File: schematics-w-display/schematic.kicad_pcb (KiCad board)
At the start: 2 copper layers, 59.8 x 61.5 mm, 8 parts, among them J1 Conn_01x21_Female, J2 Conn_01x06_Female, J3 Conn_01x21_Female, J4 Conn_01x08_Female

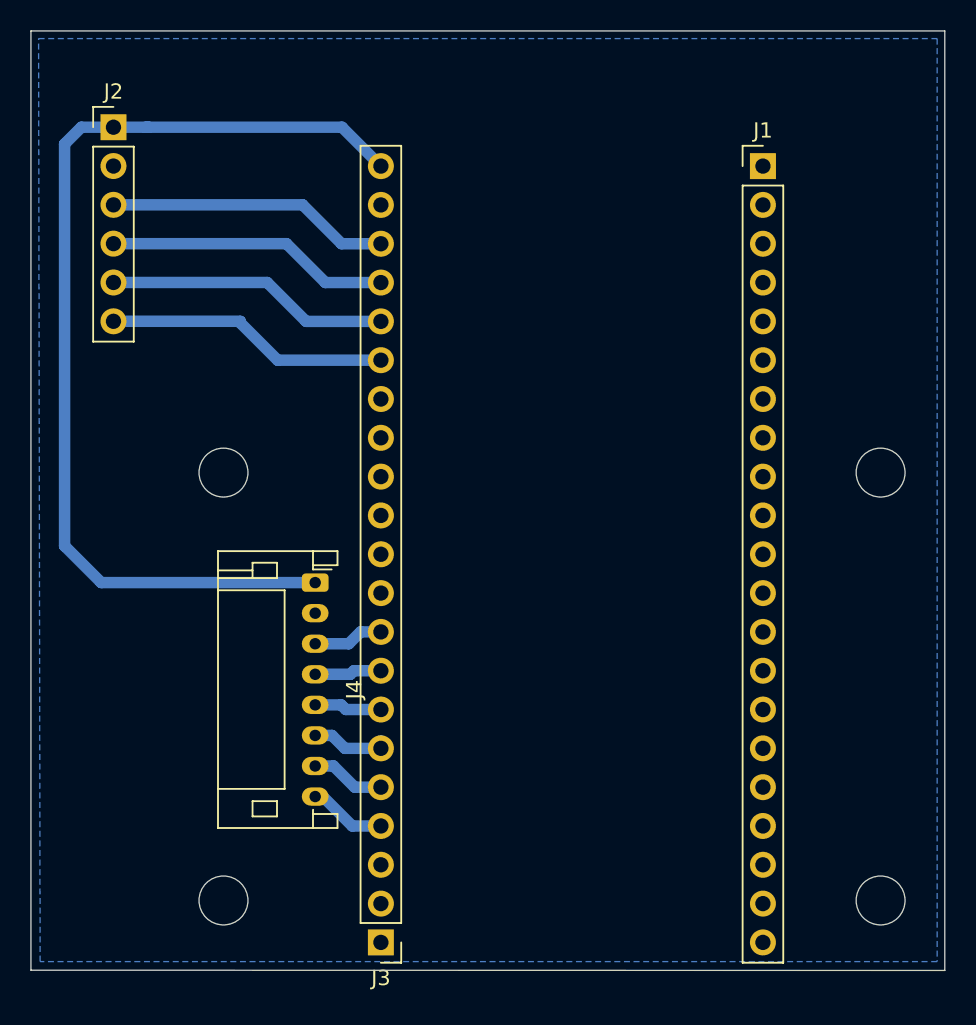
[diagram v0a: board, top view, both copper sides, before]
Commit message: Final version: again
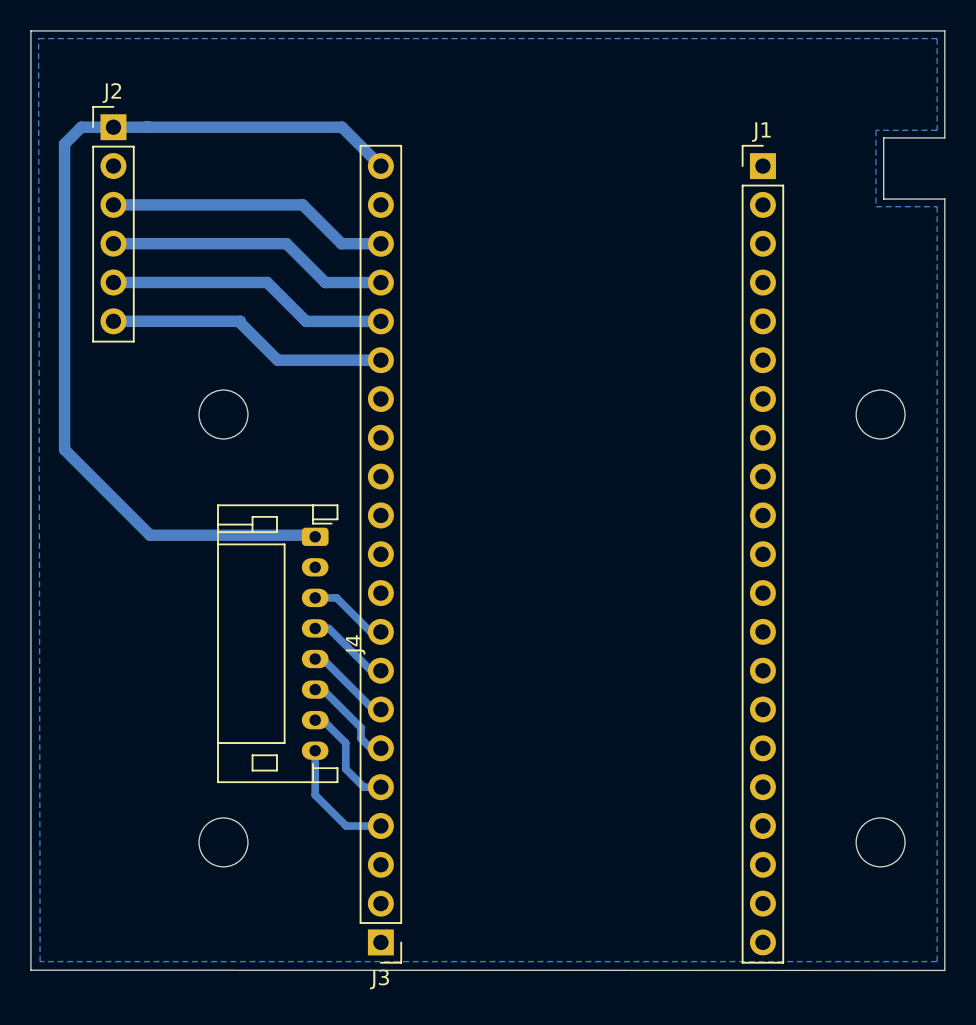
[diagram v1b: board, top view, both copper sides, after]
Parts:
- moved   3.80 mm to (99.7, 86.7)
- moved   3.80 mm to (99.7, 114.7)
- moved   3.80 mm to (142.7, 114.7)
- moved   3.80 mm to (142.7, 86.7)
- moved J4 3.00 mm to (105.7, 94.7)
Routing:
- net /3v3: track 66.1 -> 61.2 mm
- net /RST: track 4.87 -> 7.91 mm
- net /BUSY: track 5.10 -> 8.04 mm
- net /CS: track 4.70 -> 7.43 mm
- net /CLK: track 4.40 -> 6.98 mm
- net /DC: track 4.87 -> 6.98 mm
- net /MOSI: track 4.71 -> 6.56 mm
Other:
- outline, holes or cut-outs redrawn
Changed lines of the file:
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@@
   (general
     (thickness 1.6)
-    (drawings 4)
-    (tracks 43)
+    (drawings 9)
+    (tracks 58)
     (zones 0)
     (modules 8)
@@
   )
   (setup
-    (last_trace_width 0.75)
+    (last_trace_width 0.5)
+    (user_trace_width 0.5)
     (user_trace_width 0.75)
     (trace_clearance 0.2)
@@
   )
   (module Connector_JST:JST_PH_S8B-PH-K_1x08_P2.00mm_Horizontal (layer F.Cu)
-    (at 105.7 97.7 270)
+    (at 105.7 94.7 270)
     (descr "JST PH series connector, S8B-PH-K (http://www.jst-mfg.com/product/pdf/eng/ePH.pdf), generated with kicad-footprint-generator")
     (tags "connector JST PH top entry")
@@
   )
   (module MountingHole:MountingHole_3.2mm_M3 (layer F.Cu)
-    (at 99.7 90.5)
+    (at 99.7 86.7)
     (descr "Mounting Hole 3.2mm, no annular, M3")
     (tags "mounting hole 3.2mm no annular m3")
@@
   )
   (module MountingHole:MountingHole_3.2mm_M3 (layer F.Cu)
-    (at 99.7 118.5)
+    (at 99.7 114.7)
     (descr "Mounting Hole 3.2mm, no annular, M3")
     (tags "mounting hole 3.2mm no annular m3")
@@
   )
   (module MountingHole:MountingHole_3.2mm_M3 (layer F.Cu)
-    (at 142.7 118.5)
+    (at 142.7 114.7)
     (descr "Mounting Hole 3.2mm, no annular, M3")
     (tags "mounting hole 3.2mm no annular m3")
@@
   )
   (module MountingHole:MountingHole_3.2mm_M3 (layer F.Cu)
-    (at 142.7 90.5)
+    (at 142.7 86.7)
     (descr "Mounting Hole 3.2mm, no annular, M3")
     (tags "mounting hole 3.2mm no annular m3")
@@
     )
   )
+  (gr_line (start 146.9 72.6) (end 146.9 72.6) (layer Edge.Cuts) (width 0.05))
+  (gr_line (start 146.9 68.6) (end 146.9 61.6) (layer Edge.Cuts) (width 0.05))
+  (gr_line (start 142.9 72.6) (end 146.9 72.6) (layer Edge.Cuts) (width 0.05))
+  (gr_line (start 142.9 68.6) (end 142.9 72.6) (layer Edge.Cuts) (width 0.05))
+  (gr_line (start 146.9 68.6) (end 142.9 68.6) (layer Edge.Cuts) (width 0.05))
   (gr_line (start 87.1 123.063) (end 146.9 123.079) (layer Edge.Cuts) (width 0.05))
   (gr_line (start 146.9 61.6) (end 87.1 61.6) (layer Edge.Cuts) (width 0.05))
   (gr_line (start 87.1 61.6) (end 87.1 123.063) (layer Edge.Cuts) (width 0.05))
-  (gr_line (start 146.9 123.079) (end 146.9 61.6) (layer Edge.Cuts) (width 0.05))
+  (gr_line (start 146.9 123.079) (end 146.9 72.6) (layer Edge.Cuts) (width 0.05))
   (segment (start 92.5 67.9) (end 94.8 67.9) (width 0.75) (layer B.Cu) (net 1))
   (segment (start 94.8 67.9) (end 94.6 67.9) (width 0.75) (layer B.Cu) (net 1))
   (segment (start 107.455 67.9) (end 110 70.445) (width 0.75) (layer B.Cu) (net 1))
   (segment (start 94.8 67.9) (end 107.455 67.9) (width 0.75) (layer B.Cu) (net 1))
+  (segment (start 105.6 94.6) (end 105.7 94.7) (width 0.75) (layer B.Cu) (net 1))
+  (segment (start 94.9 94.6) (end 105.6 94.6) (width 0.75) (layer B.Cu) (net 1))
+  (segment (start 89.3 69) (end 89.3 89) (width 0.75) (layer B.Cu) (net 1))
+  (segment (start 89.3 89) (end 94.9 94.6) (width 0.75) (layer B.Cu) (net 1))
+  (segment (start 90.4 67.9) (end 89.3 69) (width 0.75) (layer B.Cu) (net 1))
   (segment (start 92.5 67.9) (end 90.4 67.9) (width 0.75) (layer B.Cu) (net 1))
-  (segment (start 90.4 67.9) (end 89.3 69) (width 0.75) (layer B.Cu) (net 1))
-  (segment (start 89.3 69) (end 89.3 95.3) (width 0.75) (layer B.Cu) (net 1))
-  (segment (start 91.7 97.7) (end 89.3 95.3) (width 0.75) (layer B.Cu) (net 1))
-  (segment (start 105.7 97.7) (end 91.7 97.7) (width 0.75) (layer B.Cu) (net 1))
   (segment (start 107.425 75.525) (end 110 75.525) (width 0.75) (layer B.Cu) (net 2))
   (segment (start 104.88 72.98) (end 107.425 75.525) (width 0.75) (layer B.Cu) (net 2))
@@
   (segment (start 100.8 80.7) (end 103.245 83.145) (width 0.75) (layer B.Cu) (net 5))
   (segment (start 109.935 100.9) (end 110 100.965) (width 0.75) (layer B.Cu) (net 7))
-  (segment (start 105.7 101.7) (end 107.9 101.7) (width 0.75) (layer B.Cu) (net 7))
-  (segment (start 108.675 100.925) (end 110 100.925) (width 0.75) (layer B.Cu) (net 7))
-  (segment (start 107.9 101.7) (end 108.675 100.925) (width 0.75) (layer B.Cu) (net 7))
-  (segment (start 105.7 103.7) (end 108 103.7) (width 0.75) (layer B.Cu) (net 8))
-  (segment (start 108.235 103.465) (end 110 103.465) (width 0.75) (layer B.Cu) (net 8))
-  (segment (start 108 103.7) (end 108.235 103.465) (width 0.75) (layer B.Cu) (net 8))
+  (segment (start 110 100.925) (end 109.525 100.925) (width 0.75) (layer B.Cu) (net 7))
+  (segment (start 109.225 100.925) (end 110 100.925) (width 0.25) (layer B.Cu) (net 7))
+  (segment (start 105.7 98.7) (end 107.1 98.7) (width 0.5) (layer B.Cu) (net 7))
+  (segment (start 109.325 100.925) (end 110 100.925) (width 0.5) (layer B.Cu) (net 7))
+  (segment (start 107.1 98.7) (end 109.325 100.925) (width 0.5) (layer B.Cu) (net 7))
+  (segment (start 105.7 100.7) (end 106.5 100.7) (width 0.25) (layer B.Cu) (net 8))
+  (segment (start 109.265 103.465) (end 110 103.465) (width 0.25) (layer B.Cu) (net 8))
+  (segment (start 105.7 100.7) (end 106.6 100.7) (width 0.5) (layer B.Cu) (net 8))
+  (segment (start 109.365 103.465) (end 110 103.465) (width 0.5) (layer B.Cu) (net 8))
+  (segment (start 106.6 100.7) (end 109.365 103.465) (width 0.5) (layer B.Cu) (net 8))
   (segment (start 109.805 106.2) (end 110 106.005) (width 0.75) (layer B.Cu) (net 9))
-  (segment (start 105.7 105.7) (end 107.4 105.7) (width 0.75) (layer B.Cu) (net 9))
-  (segment (start 107.705 106.005) (end 110 106.005) (width 0.75) (layer B.Cu) (net 9))
-  (segment (start 107.4 105.7) (end 107.705 106.005) (width 0.75) (layer B.Cu) (net 9))
+  (segment (start 110 106.005) (end 109.605 106.005) (width 0.75) (layer B.Cu) (net 9))
+  (segment (start 105.7 102.7) (end 106.4 102.7) (width 0.25) (layer B.Cu) (net 9))
+  (segment (start 109.705 106.005) (end 110 106.005) (width 0.25) (layer B.Cu) (net 9))
+  (segment (start 109.905 106.005) (end 110 106.005) (width 0.25) (layer B.Cu) (net 9))
+  (segment (start 105.7 102.7) (end 106.2 102.7) (width 0.5) (layer B.Cu) (net 9))
+  (segment (start 109.505 106.005) (end 110 106.005) (width 0.5) (layer B.Cu) (net 9))
+  (segment (start 106.2 102.7) (end 109.505 106.005) (width 0.5) (layer B.Cu) (net 9))
   (segment (start 109.845 108.2) (end 110 108.045) (width 0.75) (layer B.Cu) (net 10))
-  (segment (start 105.7 107.7) (end 106.8 107.7) (width 0.75) (layer B.Cu) (net 10))
-  (segment (start 107.645 108.545) (end 110 108.545) (width 0.75) (layer B.Cu) (net 10))
-  (segment (start 106.8 107.7) (end 107.645 108.545) (width 0.75) (layer B.Cu) (net 10))
-  (segment (start 105.7 109.7) (end 106.9 109.7) (width 0.75) (layer B.Cu) (net 11))
-  (segment (start 108.285 111.085) (end 110 111.085) (width 0.75) (layer B.Cu) (net 11))
-  (segment (start 106.9 109.7) (end 108.285 111.085) (width 0.75) (layer B.Cu) (net 11))
-  (segment (start 105.7 111.7) (end 106.2 111.7) (width 0.75) (layer B.Cu) (net 12))
-  (segment (start 108.125 113.625) (end 110 113.625) (width 0.75) (layer B.Cu) (net 12))
-  (segment (start 106.2 111.7) (end 108.125 113.625) (width 0.75) (layer B.Cu) (net 12))
+  (segment (start 105.7 104.7) (end 106.155 104.7) (width 0.25) (layer B.Cu) (net 10))
+  (segment (start 105.7 104.7) (end 106.2 104.7) (width 0.5) (layer B.Cu) (net 10))
+  (segment (start 106.2 104.7) (end 108.7 107.2) (width 0.5) (layer B.Cu) (net 10))
+  (segment (start 108.7 107.2) (end 108.7 107.9) (width 0.5) (layer B.Cu) (net 10))
+  (segment (start 109.345 108.545) (end 110 108.545) (width 0.5) (layer B.Cu) (net 10))
+  (segment (start 108.7 107.9) (end 109.345 108.545) (width 0.5) (layer B.Cu) (net 10))
+  (segment (start 105.7 106.7) (end 106.2 106.7) (width 0.25) (layer B.Cu) (net 11))
+  (segment (start 105.7 106.7) (end 106.5 106.7) (width 0.25) (layer B.Cu) (net 11))
+  (segment (start 106.2 106.7) (end 107.7 108.2) (width 0.5) (layer B.Cu) (net 11))
+  (segment (start 107.7 108.2) (end 107.7 109.9) (width 0.5) (layer B.Cu) (net 11))
+  (segment (start 108.885 111.085) (end 110 111.085) (width 0.5) (layer B.Cu) (net 11))
+  (segment (start 107.7 109.9) (end 108.885 111.085) (width 0.5) (layer B.Cu) (net 11))
+  (segment (start 105.7 108.7) (end 105.7 111.6) (width 0.5) (layer B.Cu) (net 12))
+  (segment (start 107.725 113.625) (end 110 113.625) (width 0.5) (layer B.Cu) (net 12))
+  (segment (start 105.7 111.6) (end 107.725 113.625) (width 0.5) (layer B.Cu) (net 12))
   (zone (net 6) (net_name GND) (layer B.Cu) (hatch edge 0.508)
     (connect_pads (clearance 0.508))
@@
     (polygon
       (pts
-        (xy 146.4 122.5) (xy 87.7 122.5) (xy 87.6 62.1) (xy 146.4 62.1)
+        (xy 146.4 68.1) (xy 142.4 68.1) (xy 142.4 73.1) (xy 146.4 73.1) (xy 146.4 122.5)
+        (xy 87.7 122.5) (xy 87.6 62.1) (xy 146.4 62.1)
       )
     )
